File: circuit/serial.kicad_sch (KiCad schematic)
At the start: 20 parts, among them J1 Port B, J2 Port C, J4 Port A, J43 Port G, Q2 2N3906, Q3 2N3906, U7 74HC04

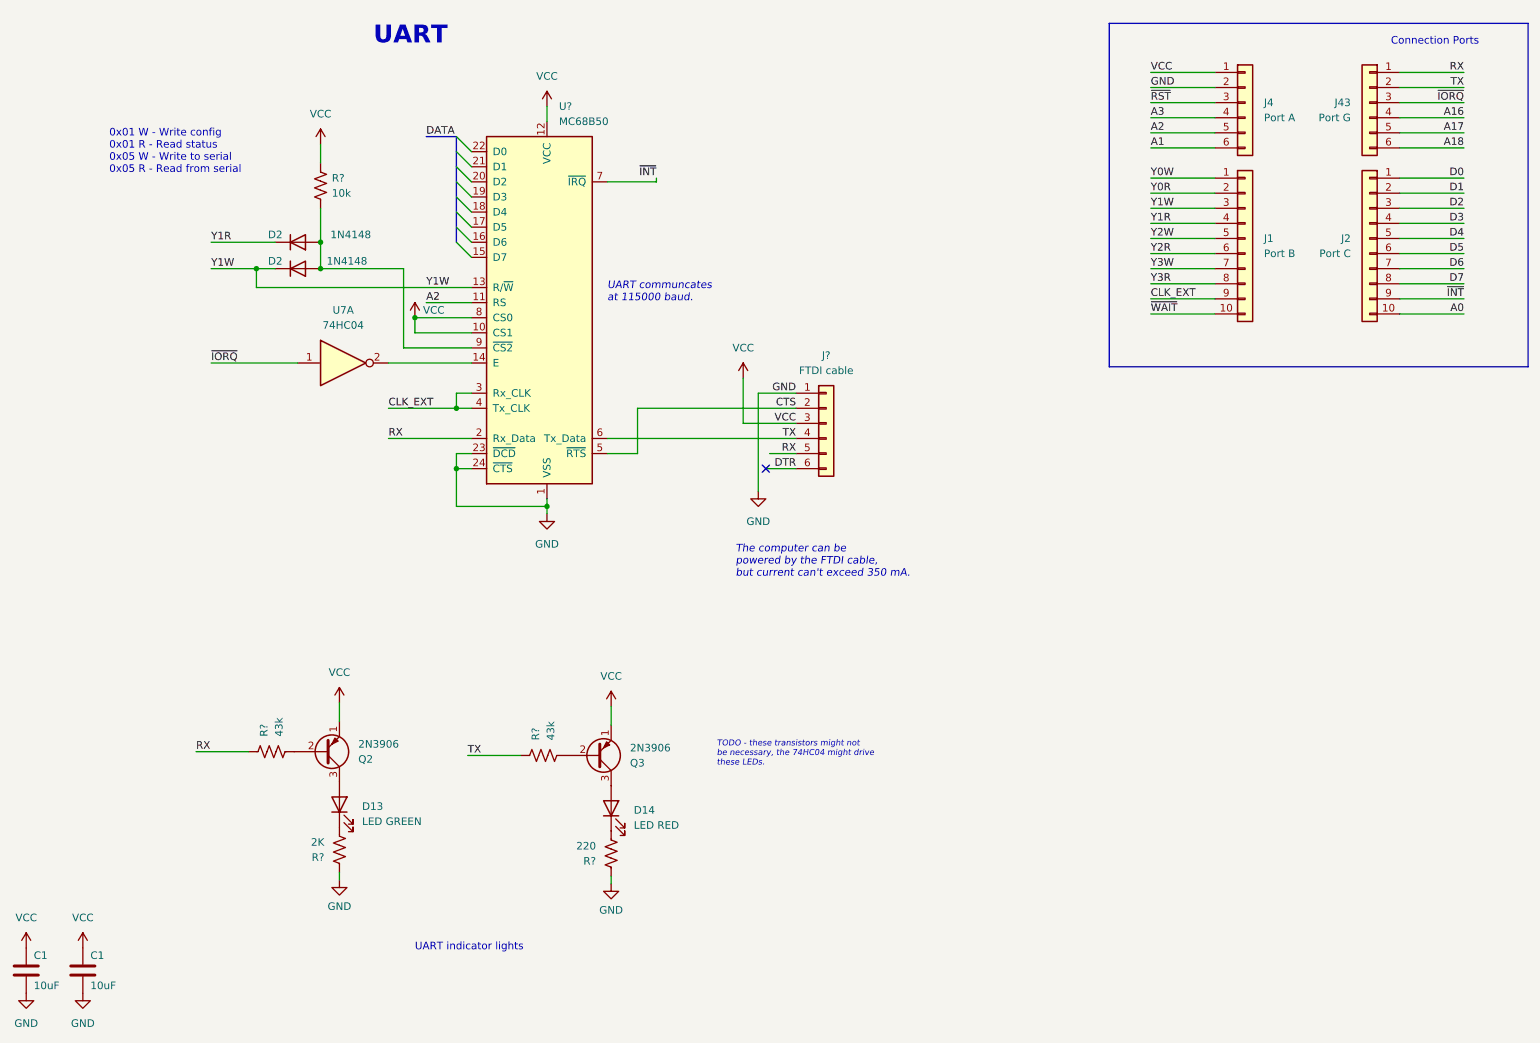
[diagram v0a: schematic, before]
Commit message: .
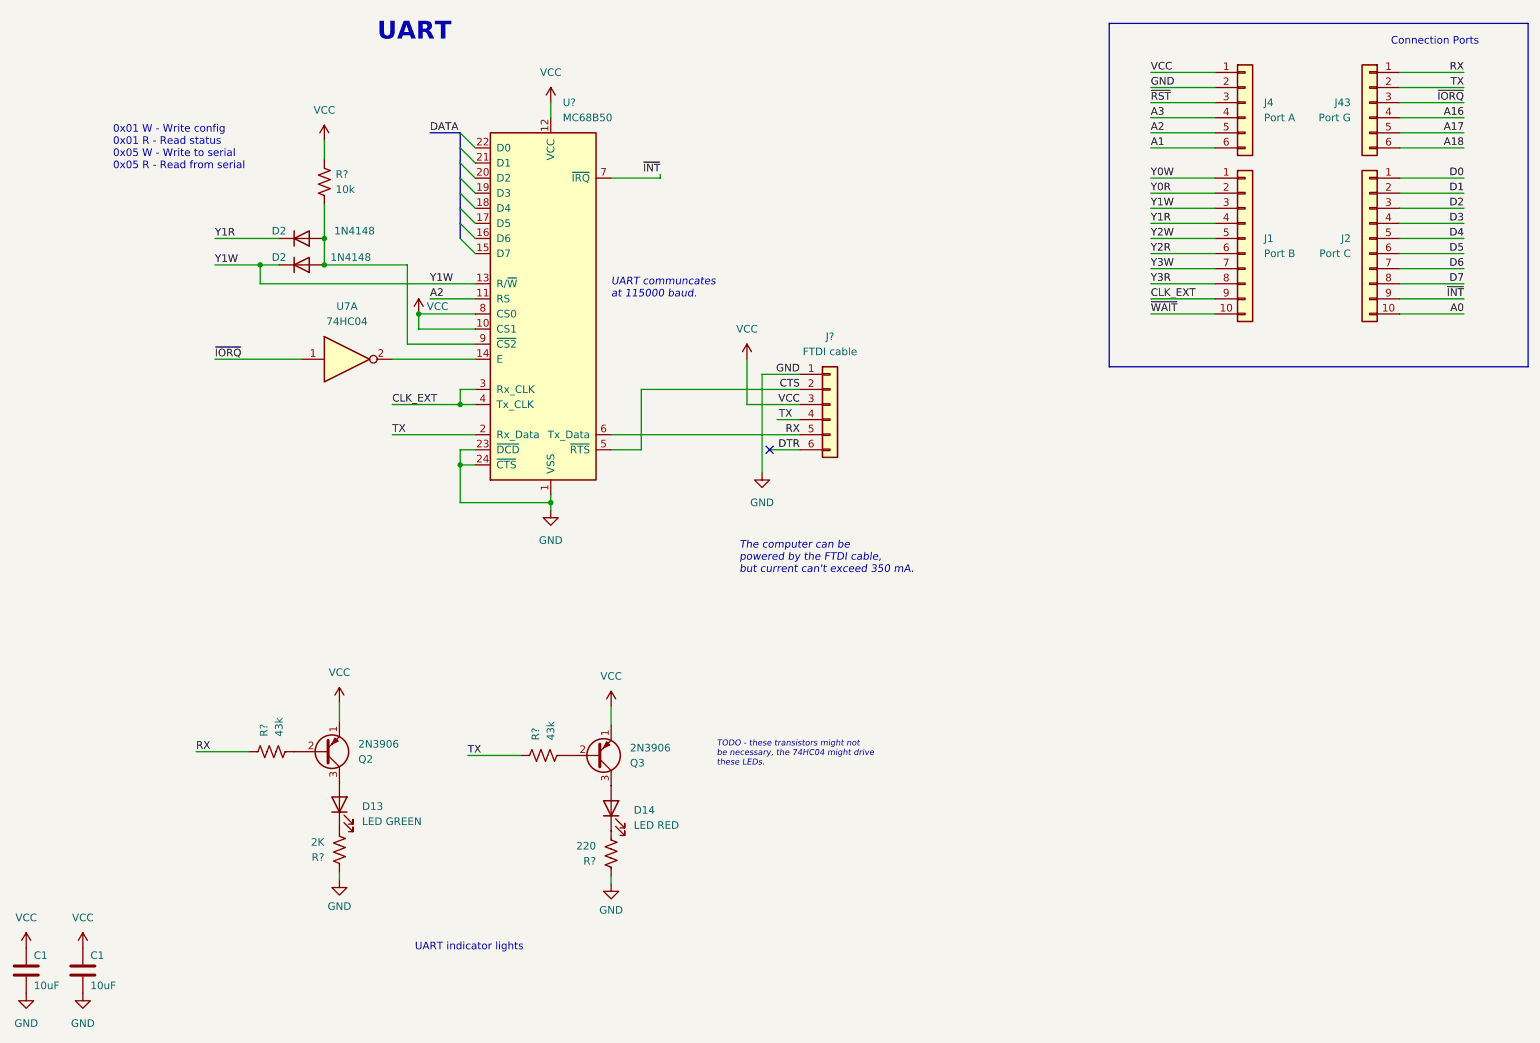
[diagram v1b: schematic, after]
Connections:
- net RX: now also U?.6 (Tx_Data); no longer U?.2 (Rx_Data)
- net TX: now also U?.2 (Rx_Data); no longer U?.6 (Tx_Data)
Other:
- moved on the sheet: D2, J?, R?, U7A, U?
